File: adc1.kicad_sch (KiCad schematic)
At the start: 57 parts, among them SW1 DRV5055A4QDBZR, SW10 DRV5055A4QDBZR, SW11 DRV5055A4QDBZR, SW12 DRV5055A4QDBZR, SW13 DRV5055A4QDBZR, SW14 DRV5055A4QDBZR, SW15 DRV5055A4QDBZR, SW16 DRV5055A4QDBZR, SW2 DRV5055A4QDBZR, SW3 DRV5055A4QDBZR, SW4 DRV5055A4QDBZR, SW5 DRV5055A4QDBZR, SW6 DRV5055A4QDBZR, SW7 DRV5055A4QDBZR, SW8 DRV5055A4QDBZR, SW9 DRV5055A4QDBZR, U2 ADS7953QDBTRQ1

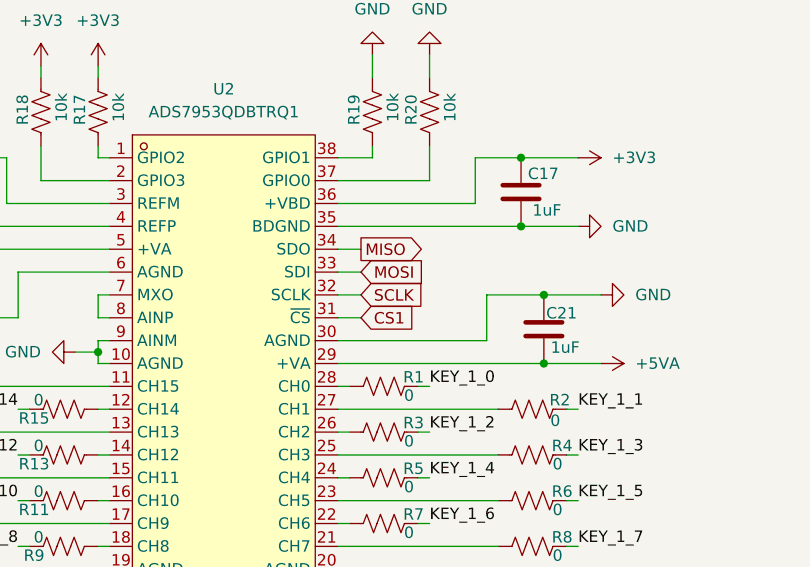
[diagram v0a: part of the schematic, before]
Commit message: hierarchical module
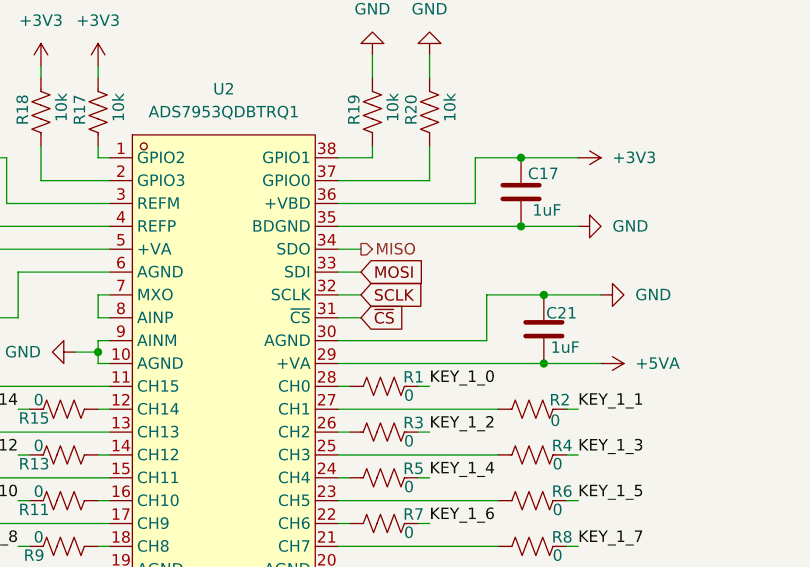
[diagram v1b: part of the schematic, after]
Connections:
- net CS1 renamed ~{CS}
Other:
- title: MUX 1 -> ADC 1
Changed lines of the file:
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@@
 	(paper "A4")
 	(title_block
-		(title "MUX 1")
+		(title "ADC 1")
 	)
 	(junction
@@
 		)
 	)
-	(global_label "CS1"
+	(global_label "~{CS}"
 		(shape input)
 		(at 132.08 120.65 0)
@@
 		)
 		(property "Intersheetrefs" "${INTERSHEET_REFS}"
-			(at 138.7542 120.65 0)
+			(at 137.5447 120.65 0)
 			(hide yes)
 			(show_name no)
@@
 		)
 	)
-	(global_label "MISO"
+	(hierarchical_label "MISO"
 		(shape output)
 		(at 132.08 113.03 0)
-		(fields_autoplaced yes)
 		(effects
 			(font
@@
 			(justify left)
 		)
-		(property "Intersheetrefs" "${INTERSHEET_REFS}"
-			(at 139.6614 113.03 0)
-			(hide yes)
-			(show_name no)
-			(do_not_autoplace no)
-			(effects
-				(font
-					(size 1.27 1.27)
-				)
-				(justify left)
-			)
-		)
 	)
 	(symbol
@@
 		(instances
 			(project "stav-keeb-65"
-				(path "/f067c205-942c-45af-b694-038ca43c147c"
-					(reference "#PWR02")
-					(unit 1)
-				)
 				(path "/f067c205-942c-45af-b694-038ca43c147c/7ed9120e-f11c-4b22-935f-1ee89d31afd6"
 					(reference "#PWR02")
@@
 		(instances
 			(project "stav-keeb-65"
-				(path "/f067c205-942c-45af-b694-038ca43c147c"
-					(reference "U2")
-					(unit 1)
-				)
 				(path "/f067c205-942c-45af-b694-038ca43c147c/7ed9120e-f11c-4b22-935f-1ee89d31afd6"
 					(reference "U2")
@@
 		(instances
 			(project "stav-keeb-65"
-				(path "/f067c205-942c-45af-b694-038ca43c147c"
-					(reference "R1")
-					(unit 1)
-				)
 				(path "/f067c205-942c-45af-b694-038ca43c147c/7ed9120e-f11c-4b22-935f-1ee89d31afd6"
 					(reference "R1")
@@
 		(instances
 			(project "stav-keeb-65"
-				(path "/f067c205-942c-45af-b694-038ca43c147c"
-					(reference "SW1")
-					(unit 1)
-				)
 				(path "/f067c205-942c-45af-b694-038ca43c147c/7ed9120e-f11c-4b22-935f-1ee89d31afd6"
 					(reference "SW1")
@@
 		(instances
 			(project "stav-keeb-65"
-				(path "/f067c205-942c-45af-b694-038ca43c147c"
-					(reference "C1")
-					(unit 1)
-				)
 				(path "/f067c205-942c-45af-b694-038ca43c147c/7ed9120e-f11c-4b22-935f-1ee89d31afd6"
 					(reference "C1")
